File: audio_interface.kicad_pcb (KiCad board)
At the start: 2 copper layers, 36 x 14 mm, 26 parts, among them IC1 ATMEGA16U2, P1 USB_A, P2 AVR-ISP, P3 OUT, P4 EAR, Q1 BC849, Q2 BC849, SW1 SW_PUSH, Y1 CSTCE16M0V53MU

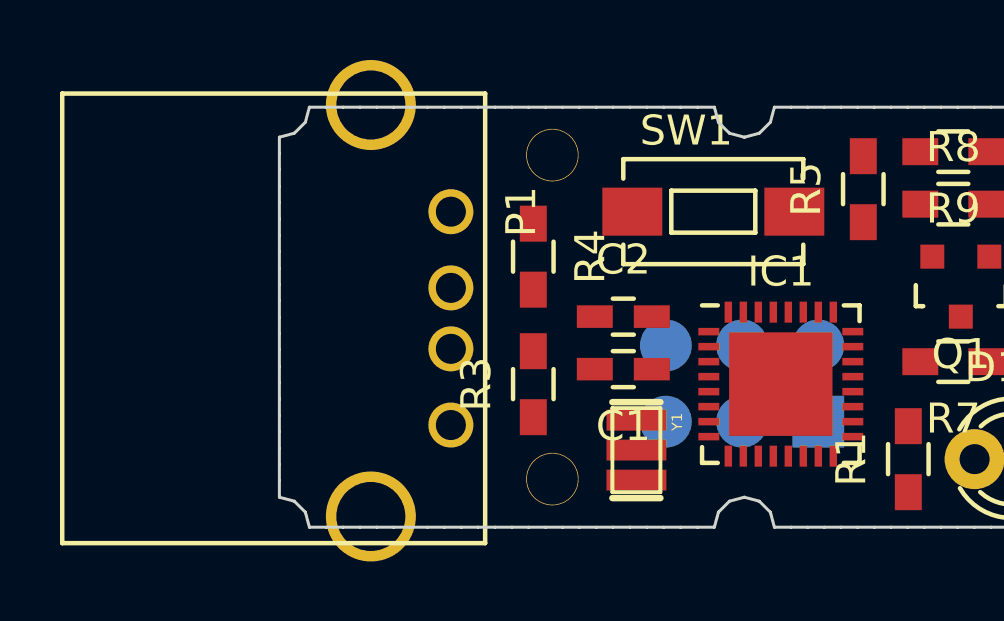
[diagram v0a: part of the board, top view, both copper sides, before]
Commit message: update
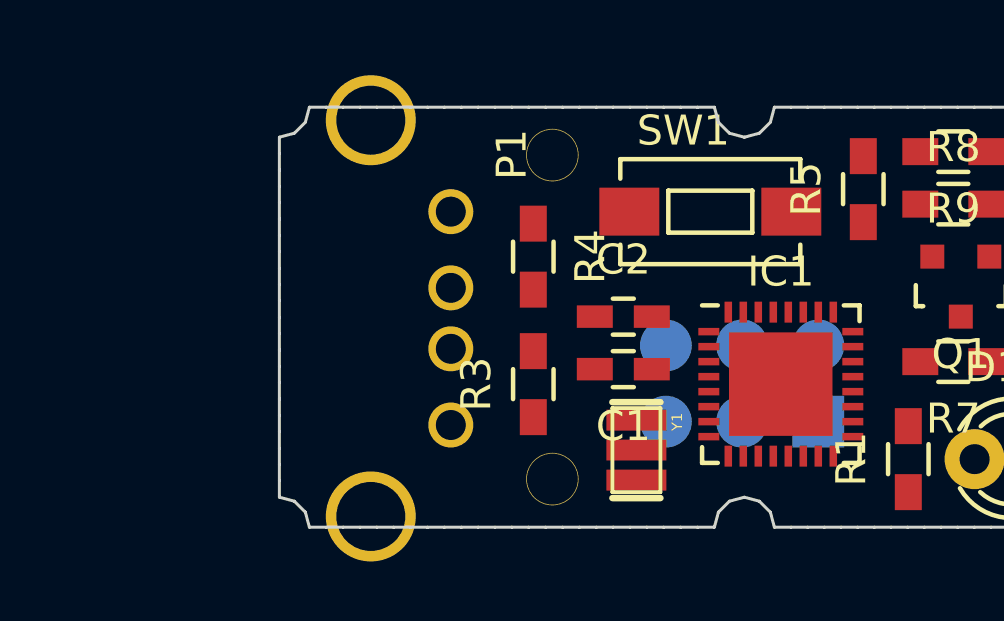
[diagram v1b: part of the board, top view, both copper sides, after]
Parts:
- P1: footprint Connect:USB_A -> KaiBader:USB_A_MALE
- moved SW1 0.10 mm to (167.4, 109.5)
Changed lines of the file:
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@@
     (links 53)
     (no_connects 53)
-    (area 145.324999 103.974999 189.286018 121.8575)
+    (area 0 0 0 0)
     (thickness 1.6)
     (drawings 0)
@@
     )
   )
-  (module Connect:USB_A (layer F.Cu)
-    (at 158.75 109.5 270)
-    (descr "USB A connector")
-    (tags "USB USB_A")
-    (fp_text reference P1 (at 0 -2.35 270) (layer F.SilkS)
-      (effects (font (size 1 1) (thickness 0.15)))
-    )
-    (fp_text value USB_A (at 3.83794 7.43458 270) (layer F.Fab)
-      (effects (font (size 1 1) (thickness 0.15)))
-    )
-    (fp_line (start -5.3 13.2) (end -5.3 -1.4) (layer F.CrtYd) (width 0.05))
-    (fp_line (start 11.95 -1.4) (end 11.95 13.2) (layer F.CrtYd) (width 0.05))
-    (fp_line (start -5.3 13.2) (end 11.95 13.2) (layer F.CrtYd) (width 0.05))
-    (fp_line (start -5.3 -1.4) (end 11.95 -1.4) (layer F.CrtYd) (width 0.05))
-    (fp_line (start 11.04986 -1.14512) (end 11.04986 12.95188) (layer F.SilkS) (width 0.15))
-    (fp_line (start -3.93614 12.95188) (end -3.93614 -1.14512) (layer F.SilkS) (width 0.15))
-    (fp_line (start 11.04986 -1.14512) (end -3.93614 -1.14512) (layer F.SilkS) (width 0.15))
-    (fp_line (start 11.04986 12.95188) (end -3.93614 12.95188) (layer F.SilkS) (width 0.15))
-    (pad 4 thru_hole circle (at 7.11286 -0.00212 180) (size 1.50114 1.50114) (drill 1.00076) (layers *.Cu *.Mask F.SilkS)
-      (net 2 GND))
-    (pad 3 thru_hole circle (at 4.57286 -0.00212 180) (size 1.50114 1.50114) (drill 1.00076) (layers *.Cu *.Mask F.SilkS)
-      (net 20 "Net-(P1-Pad3)"))
-    (pad 2 thru_hole circle (at 2.54086 -0.00212 180) (size 1.50114 1.50114) (drill 1.00076) (layers *.Cu *.Mask F.SilkS)
-      (net 21 "Net-(P1-Pad2)"))
-    (pad 1 thru_hole circle (at 0.00086 -0.00212 180) (size 1.50114 1.50114) (drill 1.00076) (layers *.Cu *.Mask F.SilkS)
-      (net 1 +5V))
-    (pad 5 thru_hole circle (at 10.16086 2.66488 180) (size 2.99974 2.99974) (drill 2.30124) (layers *.Cu *.Mask F.SilkS)
-      (net 2 GND))
-    (pad 5 thru_hole circle (at -3.55514 2.66488 180) (size 2.99974 2.99974) (drill 2.30124) (layers *.Cu *.Mask F.SilkS)
-      (net 2 GND))
-    (model Connect.3dshapes/USB_A.wrl
-      (at (xyz 0.14 0 0))
-      (scale (xyz 1 1 1))
-      (rotate (xyz 0 0 90))
-    )
-  )
   (module KaiBader:Pin_Header_SMD_2x03 (layer B.Cu)
     (at 171 116.5 90)
@@
   )
   (module Buttons_Switches_SMD:SW_SPST_EVQPE1 (layer F.Cu)
-    (at 167.5 109.5)
+    (at 167.4 109.5)
     (descr "Light Touch Switch")
     (attr smd)
@@
     (pad "" thru_hole circle (at 9.1 -1.6) (size 1.75 1.75) (drill 1.7) (layers *.Cu *.Mask F.SilkS))
   )
+  (module KaiBader:USB_A_MALE (layer F.Cu)
+    (at 158.75 109.5 270)
+    (descr "USB A connector")
+    (tags "USB USB_A")
+    (fp_text reference P1 (at -1.905 -2.032 270) (layer F.SilkS)
+      (effects (font (size 1 1) (thickness 0.15)))
+    )
+    (fp_text value USB_A (at 3.556 2.667 270) (layer F.Fab)
+      (effects (font (size 1 1) (thickness 0.15)))
+    )
+    (fp_line (start -4.064 13.081) (end 11.176 13.081) (layer F.CrtYd) (width 0.1))
+    (fp_line (start 11.176 13.081) (end 11.176 -1.27) (layer F.CrtYd) (width 0.1))
+    (fp_line (start 11.176 -1.27) (end -4.064 -1.27) (layer F.CrtYd) (width 0.1))
+    (fp_line (start -4.064 -1.27) (end -4.064 13.081) (layer F.CrtYd) (width 0.1))
+    (pad 4 thru_hole circle (at 7.112 0 180) (size 1.5 1.5) (drill 1) (layers *.Cu *.Mask F.SilkS)
+      (net 2 GND))
+    (pad 3 thru_hole circle (at 4.572 0 180) (size 1.5 1.5) (drill 1) (layers *.Cu *.Mask F.SilkS)
+      (net 20 "Net-(P1-Pad3)"))
+    (pad 2 thru_hole circle (at 2.54 0 180) (size 1.5 1.5) (drill 1) (layers *.Cu *.Mask F.SilkS)
+      (net 21 "Net-(P1-Pad2)"))
+    (pad 1 thru_hole circle (at 0 0 180) (size 1.5 1.5) (drill 1) (layers *.Cu *.Mask F.SilkS)
+      (net 1 +5V))
+    (pad 5 thru_hole circle (at 10.16 2.667 180) (size 3 3) (drill 2.3) (layers *.Cu *.Mask F.SilkS)
+      (net 2 GND))
+    (pad 5 thru_hole circle (at -3.048 2.667 180) (size 3 3) (drill 2.3) (layers *.Cu *.Mask F.SilkS)
+      (net 2 GND))
+    (model Connect.3dshapes/USB_A.wrl
+      (at (xyz 0.14 0 0))
+      (scale (xyz 1 1 1))
+      (rotate (xyz 0 0 90))
+    )
+  )
 )

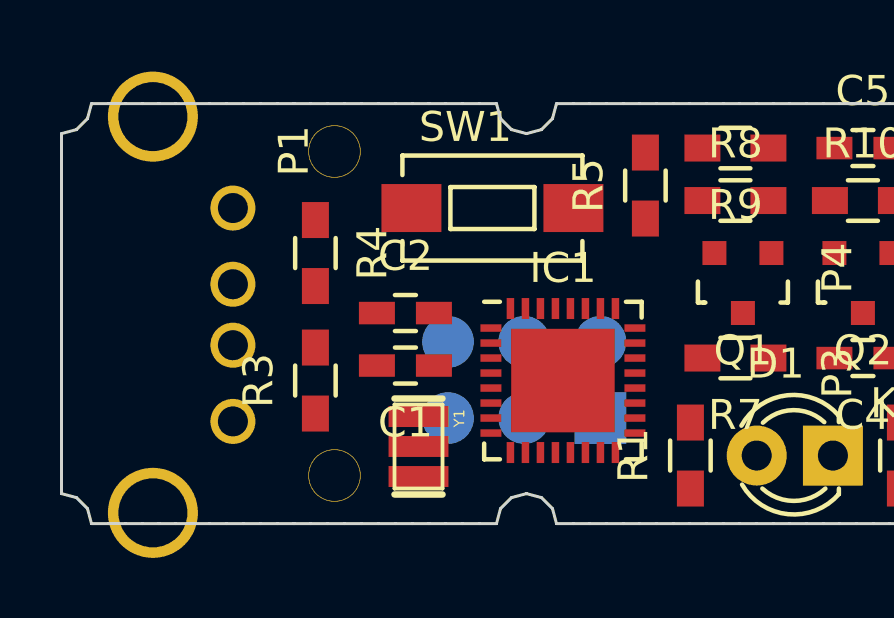
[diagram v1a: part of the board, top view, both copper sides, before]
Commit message: update
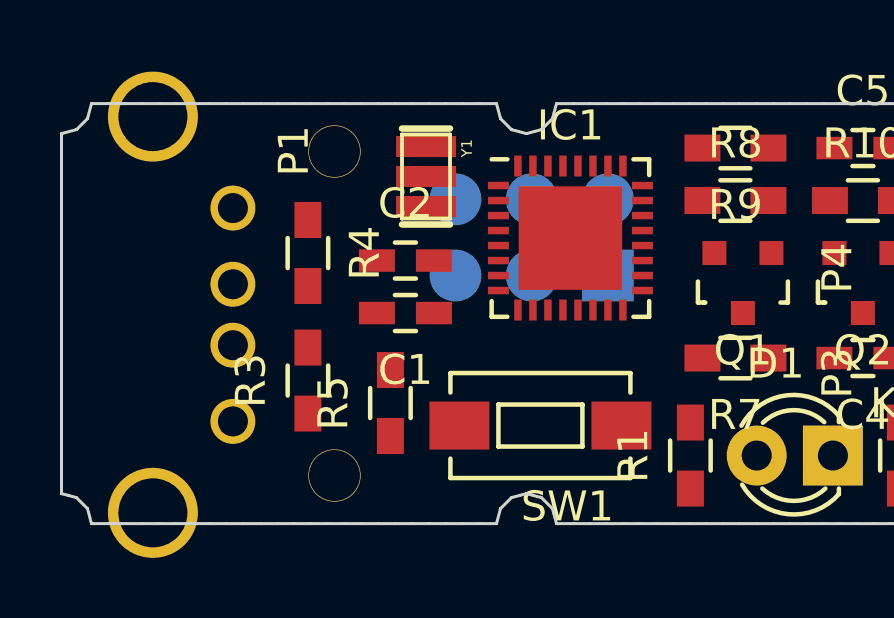
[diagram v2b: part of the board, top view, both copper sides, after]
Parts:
- moved R5 11.2 mm to (164.0, 116.0)
- moved Y1 9.00 mm to (163.5, 107.0)
- moved SW1 7.42 mm to (169.0, 116.8), turned to 180 degrees
- moved IC1 4.76 mm to (170.0, 110.5)
- moved P2 4.76 mm to (171.2, 111.8)
- moved C1 1.75 mm to (164.5, 113.0)
- moved C2 1.75 mm to (164.5, 111.2)
- moved R3 0.25 mm to (161.2, 115.2)
- moved R4 0.25 mm to (161.2, 111.0)
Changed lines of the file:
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@@
     (links 53)
     (no_connects 53)
-    (area 0 0 0 0)
+    (area 145.418999 104.3075 189.286018 121.8575)
     (thickness 1.6)
     (drawings 0)
@@
   )
   (module Capacitors_SMD:C_0603_HandSoldering (layer F.Cu)
-    (at 164.5 114.75 180)
+    (at 164.5 113 180)
     (descr "Capacitor SMD 0603, hand soldering")
     (tags "capacitor 0603")
@@
   )
   (module Capacitors_SMD:C_0603_HandSoldering (layer F.Cu)
-    (at 164.5 113)
+    (at 164.5 111.25)
     (descr "Capacitor SMD 0603, hand soldering")
     (tags "capacitor 0603")
@@
   )
   (module Housings_DFN_QFN:QFN-32-1EP_5x5mm_Pitch0.5mm (layer F.Cu)
-    (at 169.75 115.25)
+    (at 170 110.5)
     (descr "UH Package; 32-Lead Plastic QFN (5mm x 5mm); (see Linear Technology QFN_32_05-08-1693.pdf)")
     (tags "QFN 0.5")
@@
   )
   (module KaiBader:Pin_Header_SMD_2x03 (layer B.Cu)
-    (at 171 116.5 90)
+    (at 171.25 111.75 90)
     (descr "Through hole pin header")
     (tags "pin header")
@@
   )
   (module Resistors_SMD:R_0603_HandSoldering (layer F.Cu)
-    (at 161.5 115.25 90)
+    (at 161.25 115.25 90)
     (descr "Resistor SMD 0603, hand soldering")
     (tags "resistor 0603")
@@
   )
   (module Resistors_SMD:R_0603_HandSoldering (layer F.Cu)
-    (at 161.5 111 270)
+    (at 161.25 111 270)
     (descr "Resistor SMD 0603, hand soldering")
     (tags "resistor 0603")
@@
   )
   (module Resistors_SMD:R_0603_HandSoldering (layer F.Cu)
-    (at 172.5 108.75 90)
+    (at 164 116 90)
     (descr "Resistor SMD 0603, hand soldering")
     (tags "resistor 0603")
@@
   )
   (module Buttons_Switches_SMD:SW_SPST_EVQPE1 (layer F.Cu)
-    (at 167.4 109.5)
+    (at 169 116.75 180)
     (descr "Light Touch Switch")
     (attr smd)
-    (fp_text reference SW1 (at -0.9 -2.7) (layer F.SilkS)
-      (effects (font (size 1 1) (thickness 0.15)))
-    )
-    (fp_text value SW_PUSH (at 0 0) (layer F.Fab)
+    (fp_text reference SW1 (at -0.9 -2.7 180) (layer F.SilkS)
+      (effects (font (size 1 1) (thickness 0.15)))
+    )
+    (fp_text value SW_PUSH (at 0 0 180) (layer F.Fab)
       (effects (font (size 1 1) (thickness 0.15)))
     )
@@
     (fp_line (start 3 -1.75) (end -3 -1.75) (layer F.SilkS) (width 0.15))
     (fp_line (start -3 1.75) (end 3 1.75) (layer F.SilkS) (width 0.15))
-    (pad 2 smd rect (at 2.7 0) (size 2 1.6) (layers F.Cu F.Paste F.Mask)
+    (pad 2 smd rect (at 2.7 0 180) (size 2 1.6) (layers F.Cu F.Paste F.Mask)
       (net 17 ~RESET))
-    (pad 1 smd rect (at -2.7 0) (size 2 1.6) (layers F.Cu F.Paste F.Mask)
+    (pad 1 smd rect (at -2.7 0 180) (size 2 1.6) (layers F.Cu F.Paste F.Mask)
       (net 2 GND))
   )
   (module KaiBader:CSTCE16M0V53 (layer F.Cu)
-    (at 163.25 116 270)
+    (at 163.5 107 270)
     (descr "CSTCE16M0V53 CERAMIC RESONATOR (CERALOCK) 16 MHZ CHIP TYPE")
     (tags "CSTCE16M0V53 CERAMIC RESONATOR (CERALOCK) 16 MHZ CHIP TYPE")

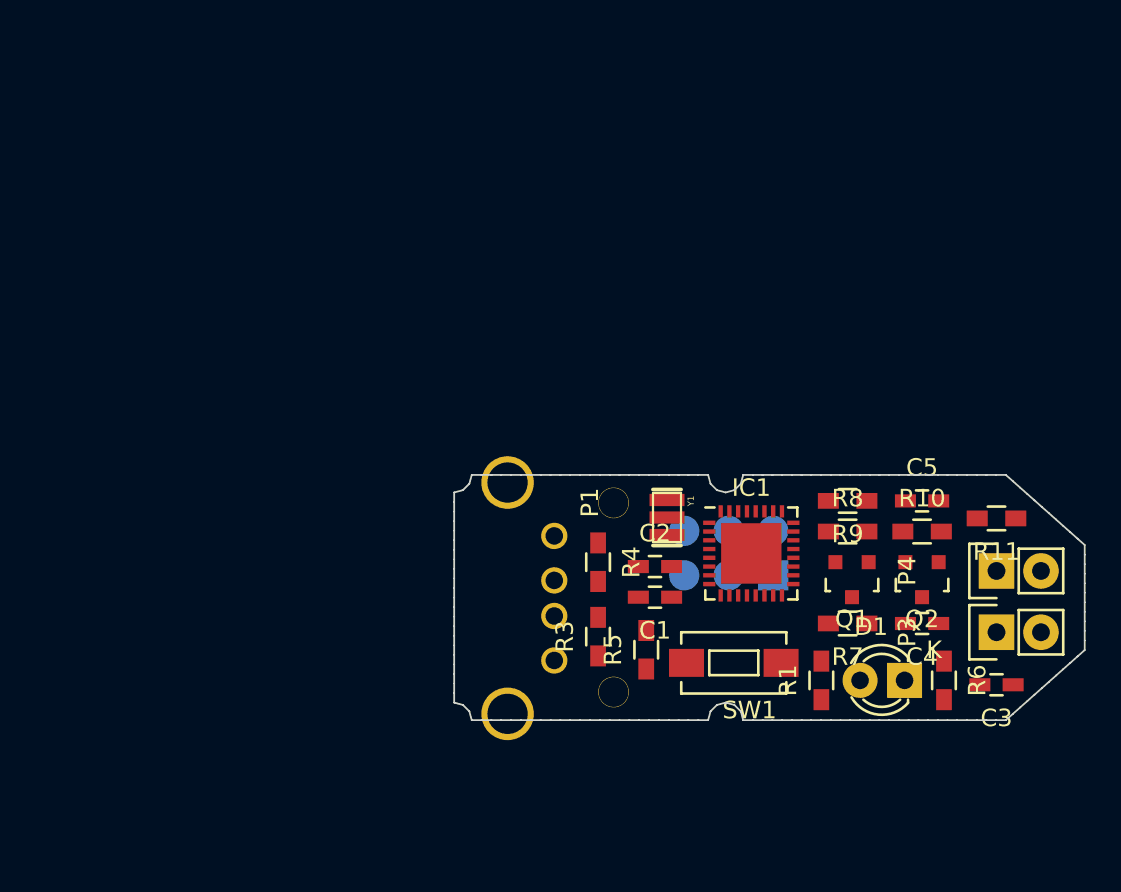
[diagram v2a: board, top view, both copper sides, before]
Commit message: update
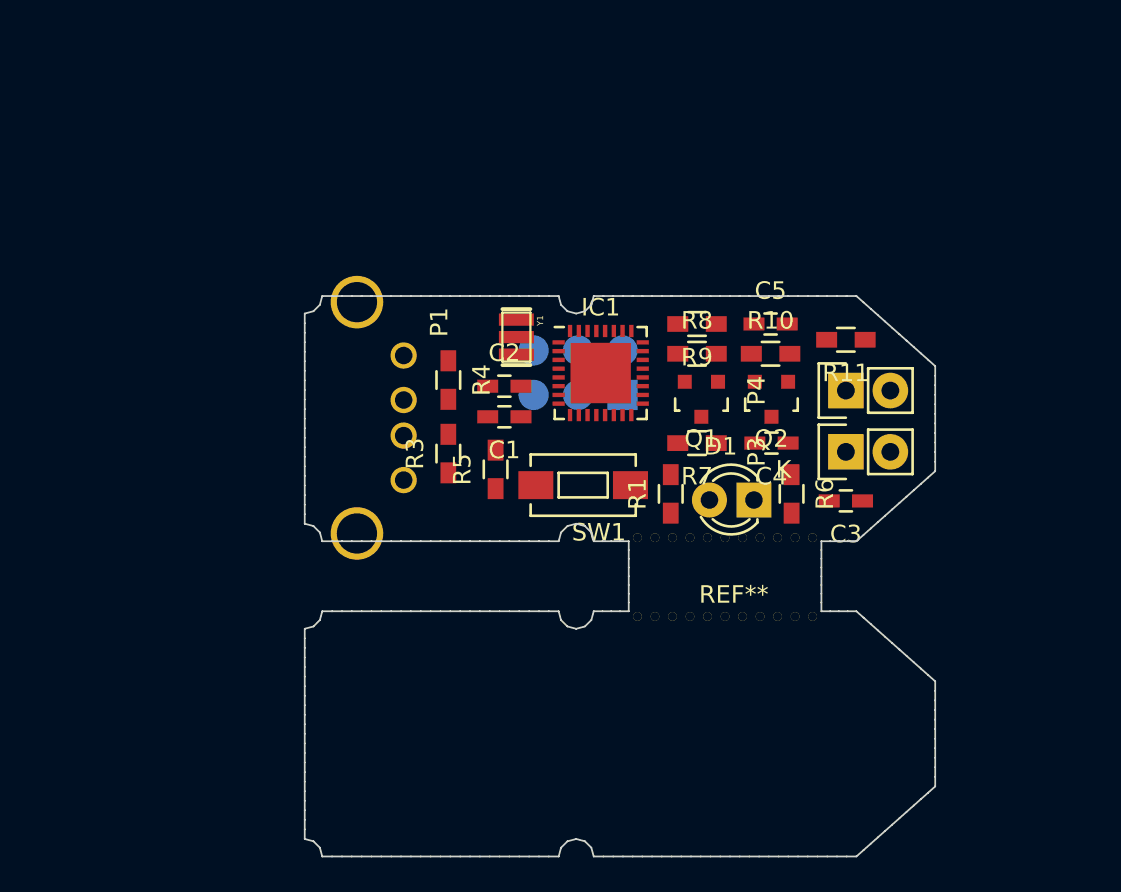
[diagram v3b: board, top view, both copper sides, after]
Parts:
- removed ?: AK-S-27 Case, KaiBader:AK-S-27_Case
- added REF**: Mousebites, KaiBader:Mousebites, F.Cu at (163.5, 114.1)
- moved R6 13.8 mm to (172.3, 107.1)
- moved R1 13.7 mm to (165.4, 107.1)
- moved C3 13.6 mm to (175.4, 107.5)
- moved R3 13.5 mm to (152.7, 104.8)
- moved R4 13.5 mm to (152.7, 100.6)
- moved C1 13.4 mm to (155.9, 102.7)
- moved C2 13.4 mm to (155.9, 101.0)
- moved C4 13.4 mm to (171.2, 104.2)
- moved D1 13.4 mm to (170.2, 107.5)
- moved IC1 13.4 mm to (161.4, 100.2)
- moved P1 13.4 mm to (150.2, 99.2)
- moved P2 13.4 mm to (162.7, 101.5)
- moved P3 13.4 mm to (175.4, 104.7)
- moved P4 13.4 mm to (175.4, 101.2)
- moved Q1 13.4 mm to (167.2, 101.7)
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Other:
- board size 36 x 14 mm -> 36 x 32 mm

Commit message: update
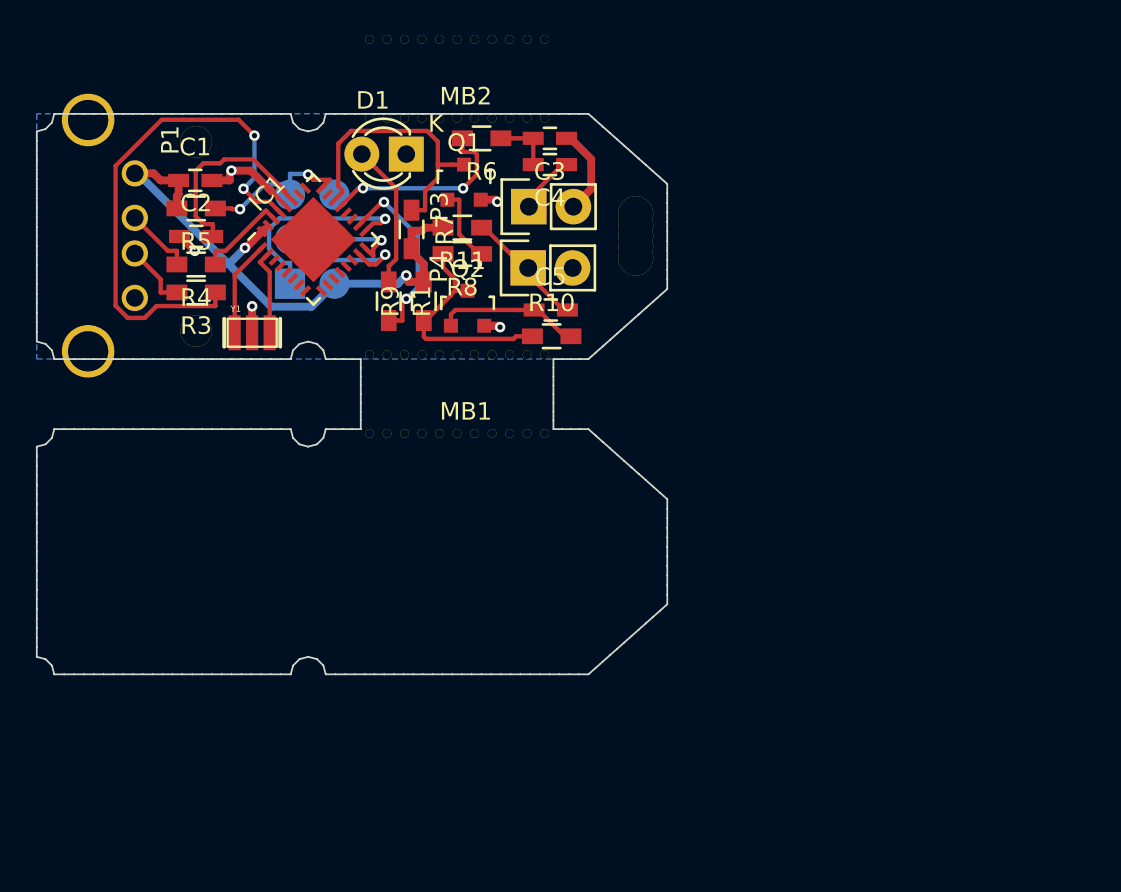
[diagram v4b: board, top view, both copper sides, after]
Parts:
- removed SW1: SW_PUSH, Buttons_Switches_SMD:SW_SPST_EVQPE1
- added MB2: Mousebites, KaiBader:Mousebites, F.Cu at (148.2, 85.7)
- added REF**: Strain_Relief, KaiBader:Strain_Relief, F.Cu at (163.4, 91.1)
- added Ref**: AK-S-27 Mount, KaiBader:AK-S-27_Mount, F.Cu at (129.2, 99.4)
- moved D1 28.0 mm to (150.3, 87.7)
- moved R6 26.9 mm to (154.6, 86.8), turned to 180 degrees
- moved C3 26.7 mm to (158.5, 86.8)
- moved P3 22.9 mm to (157.3, 90.7)
- moved R11 22.8 mm to (153.5, 91.9)
- moved R5 22.7 mm to (138.3, 90.8), turned to 180 degrees
- moved C1 22.2 mm to (138.2, 89.2), turned to 0 degrees
- moved R7 20.4 mm to (150.6, 92.0), turned to 270 degrees
- moved C4 20.3 mm to (158.5, 88.3)
- moved P2 20.0 mm to (143.7, 95.1), turned to 0 degrees
- moved C2 19.6 mm to (138.3, 92.4)
- moved R1 19.5 mm to (149.3, 96.1), turned to 270 degrees
- moved P4 19.4 mm to (157.3, 94.2)
- moved P1 18.5 mm to (134.8, 88.8)
- moved MB1 18.5 mm to (148.2, 103.7)
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- renumbered REF** to MB1
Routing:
- net +5V: track 0.00 -> 33.3 mm, vias 0 -> 2
- net Net-(IC1-Pad29): track 0.00 -> 30.4 mm, vias 0 -> 2
- net GND: track 0.00 -> 16.3 mm, vias 0 -> 5
- net PC7: track 0.00 -> 16.3 mm
- net Net-(Q2-Pad3): track 0.00 -> 12.9 mm
- net MISO: track 0.00 -> 12.2 mm, vias 0 -> 1
- net PD0: track 0.00 -> 11.4 mm, vias 0 -> 2
- net Net-(C2-Pad2): track 0.00 -> 11.3 mm
- net PB4: track 0.00 -> 10.7 mm, vias 0 -> 2
- net ~RESET: track 0.00 -> 9.15 mm, vias 0 -> 2
- net Net-(C5-Pad2): track 0.00 -> 8.56 mm
- net Net-(D1-Pad2): track 0.00 -> 8.31 mm
- net SCK: track 0.00 -> 8.29 mm, vias 0 -> 1
- net Net-(C5-Pad1): track 0.00 -> 8.23 mm
- net Net-(IC1-Pad1): track 0.00 -> 5.51 mm
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- added copper zone on B.Cu, net GND
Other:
- net class PWR added: clearance 0.2, trace_width 0.45, via_dia 0.6, via_drill 0.4
